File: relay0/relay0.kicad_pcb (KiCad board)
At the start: 2 copper layers, 15 parts, among them J1 2601-1106, J2 2601-1106, J3 2601-1102, K1 J107F1AS2012VDC.80, K2 J107F1AS2012VDC.80, K3 J107F1AS2012VDC.80, K4 J107F1AS2012VDC.80, K5 J107F1AS2012VDC.80, K6 J107F1AS2012VDC.80

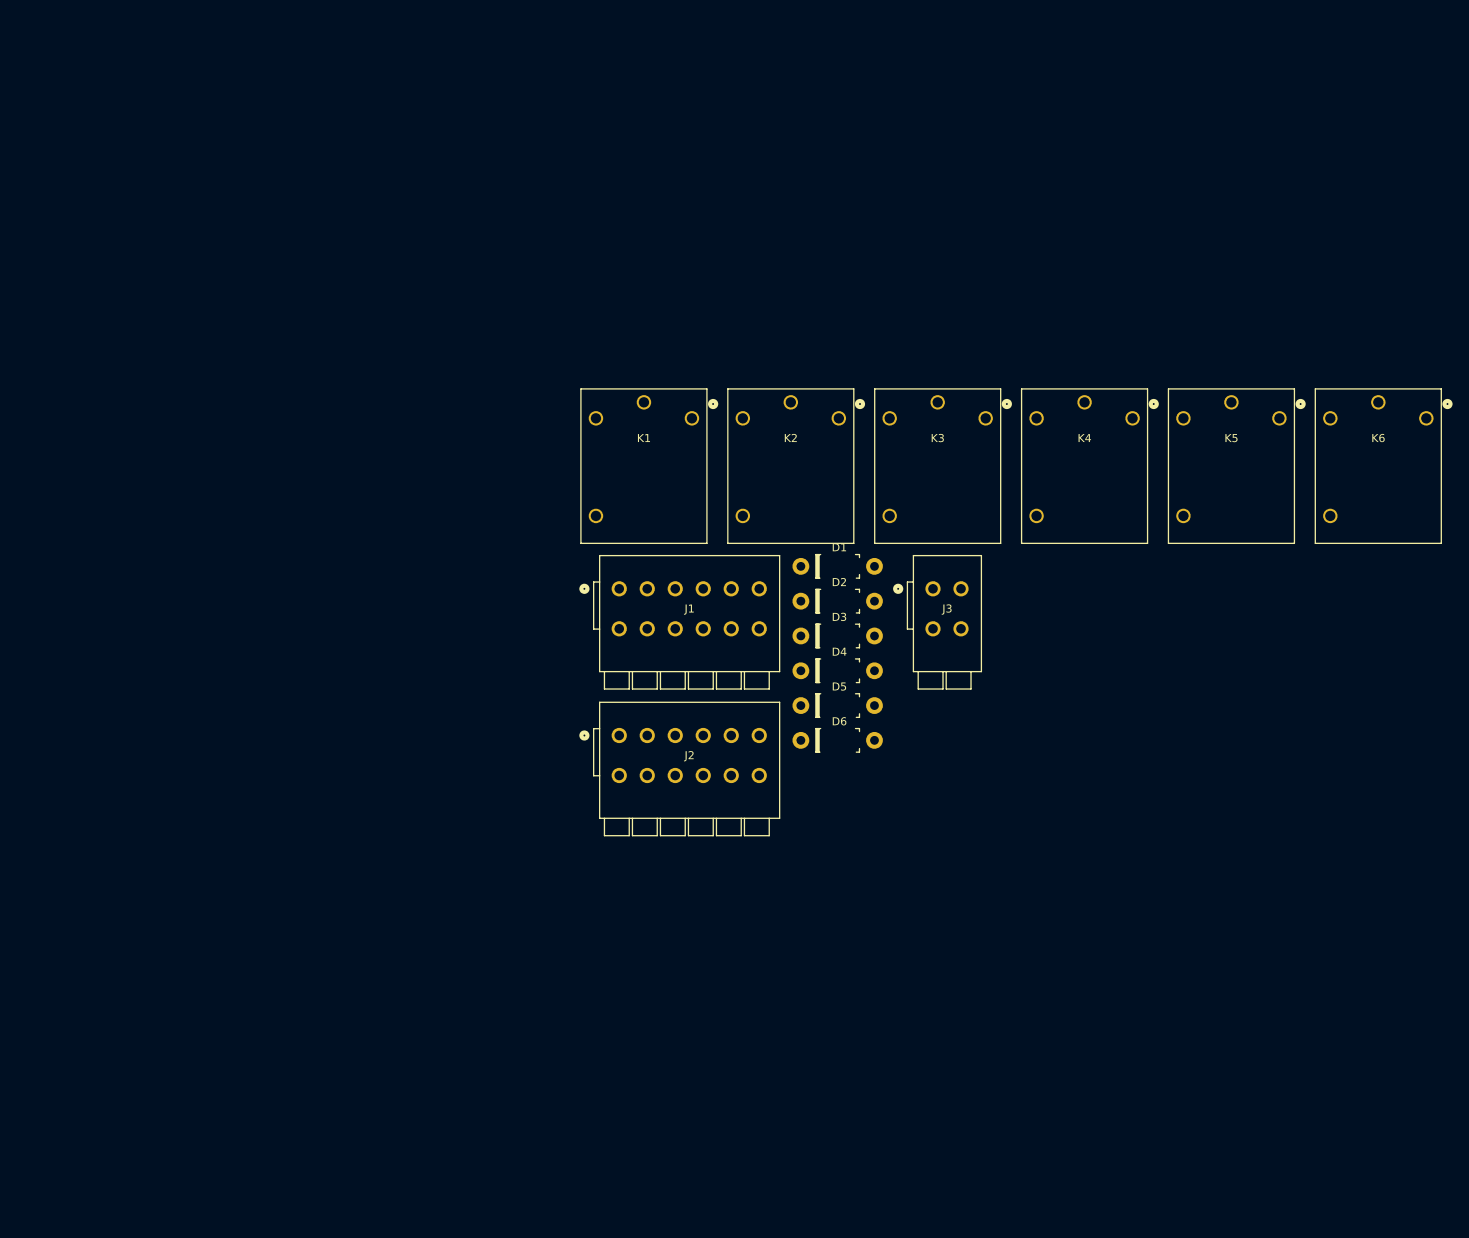
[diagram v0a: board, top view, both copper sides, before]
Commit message: PCB Design updates
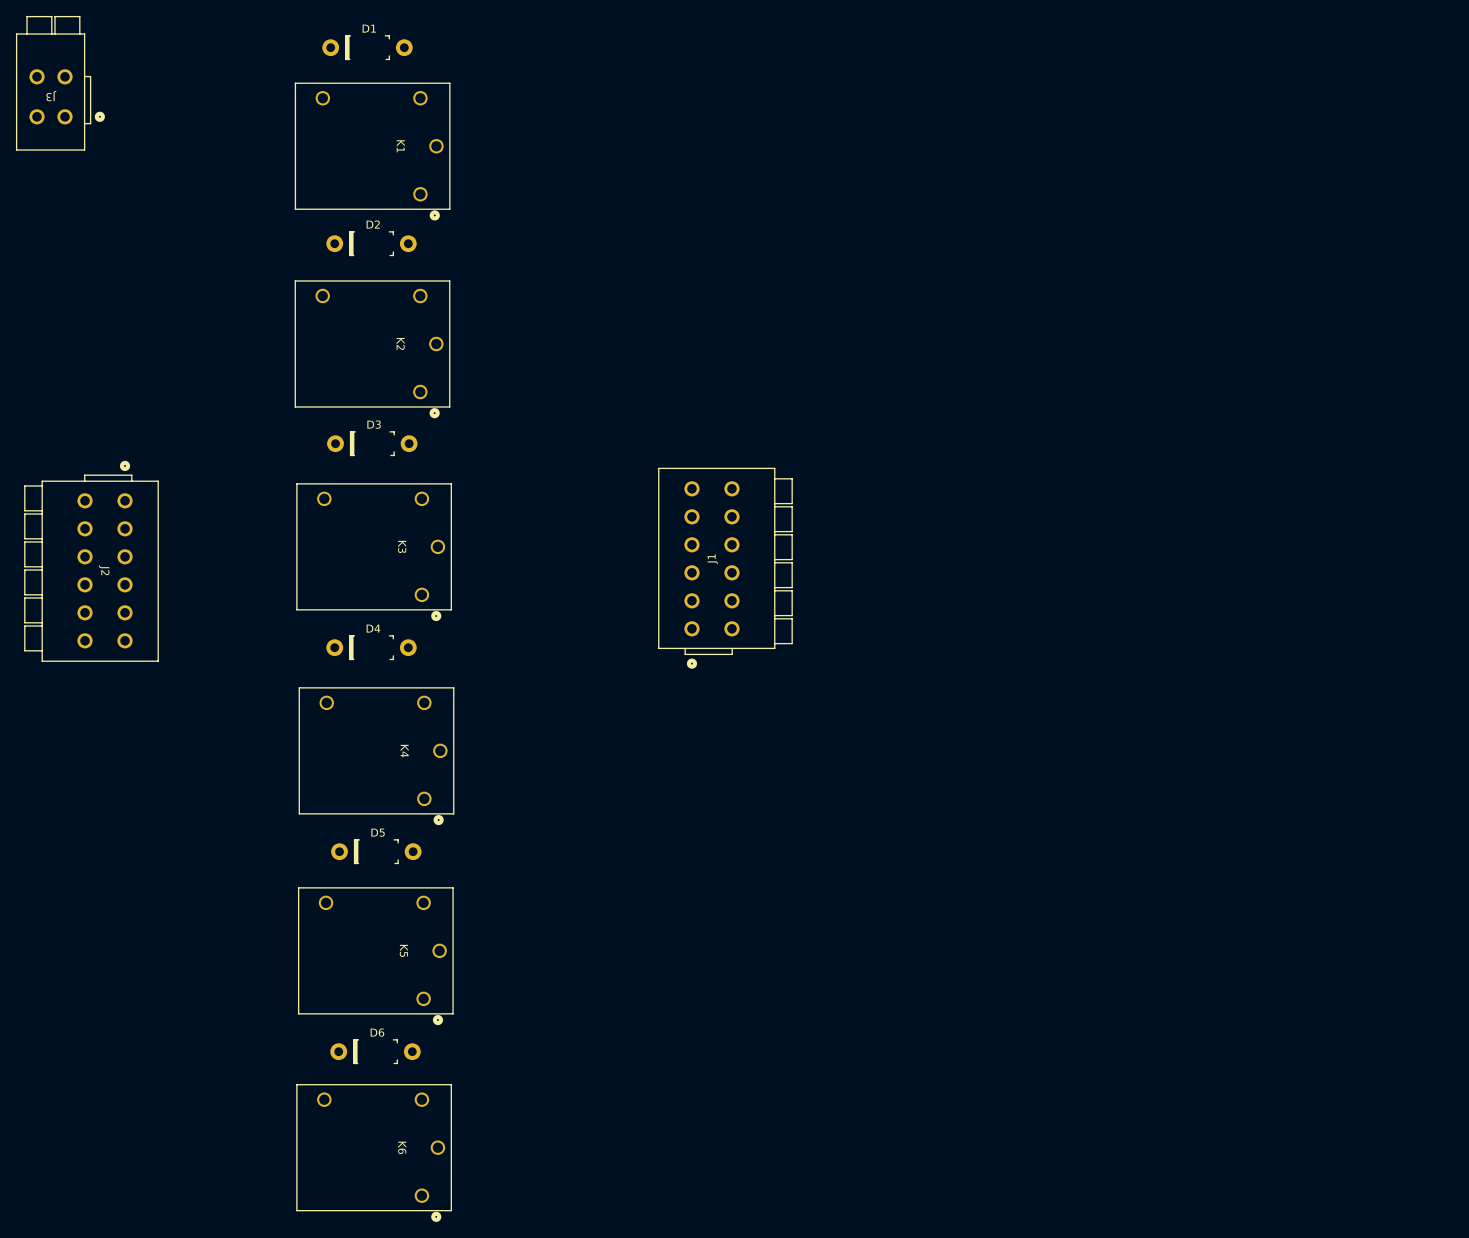
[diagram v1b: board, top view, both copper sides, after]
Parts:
- moved K6 150.0 mm to (66.1, 154.4), turned to -90 degrees
- moved J3 123.5 mm to (19.5, 25.5), turned to 180 degrees
- moved K5 120.4 mm to (66.3, 129.8), turned to -90 degrees
- moved K4 91.6 mm to (66.4, 104.8), turned to -90 degrees
- moved D1 87.5 mm to (52.7, 16.9)
- moved D2 73.4 mm to (53.2, 41.4)
- moved D6 69.7 mm to (53.7, 142.4)
- moved J2 68.4 mm to (27.0, 73.5), turned to -90 degrees
- moved K3 65.0 mm to (66.1, 79.3), turned to -90 degrees
- moved D3 62.9 mm to (53.3, 66.4)
- moved D5 60.5 mm to (53.8, 117.4)
- moved D4 58.3 mm to (53.2, 91.9)
- moved K2 44.9 mm to (65.9, 53.9), turned to -90 degrees
- moved K1 41.2 mm to (65.9, 29.2), turned to -90 degrees
- moved J1 10.4 mm to (97.9, 89.5), turned to 90 degrees
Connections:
- D1 pad A: Net-(D1-PadA) -> Net-(J3-2_1)
- D2 pad A: Net-(D2-PadA) -> Net-(J3-2_1)
- D2 pad K: Net-(D1-PadA) -> Net-(J3-1_1)
- D3 pad A: Net-(D3-PadA) -> Net-(J3-2_1)
- D3 pad K: Net-(D2-PadA) -> Net-(J3-1_1)
- D4 pad A: Net-(D4-PadA) -> Net-(J3-2_1)
- D4 pad K: Net-(D3-PadA) -> Net-(J3-1_1)
- D5 pad A: Net-(D5-PadA) -> Net-(J3-2_1)
- D5 pad K: Net-(D4-PadA) -> Net-(J3-1_1)
- D6 pad K: Net-(D5-PadA) -> Net-(J3-1_1)
- J2 pad 7: Net-(J2-4_1) -> Net-(J2-2_1)
- J2 pad 8: Net-(J2-4_1) -> Net-(J2-2_1)
- K1 pad 2: Net-(D1-PadA) -> Net-(J3-2_1)
- K2 pad 2: Net-(D2-PadA) -> Net-(J3-2_1)
- K2 pad 4: Net-(D1-PadA) -> Net-(J3-1_1)
- K3 pad 2: Net-(D3-PadA) -> Net-(J3-2_1)
- K3 pad 4: Net-(D2-PadA) -> Net-(J3-1_1)
- K4 pad 2: Net-(D4-PadA) -> Net-(J3-2_1)
- K4 pad 3: Net-(J2-4_1) -> Net-(J2-2_1)
- K4 pad 4: Net-(D3-PadA) -> Net-(J3-1_1)
- K5 pad 2: Net-(D5-PadA) -> Net-(J3-2_1)
- K5 pad 4: Net-(D4-PadA) -> Net-(J3-1_1)
- K6 pad 4: Net-(D5-PadA) -> Net-(J3-1_1)
